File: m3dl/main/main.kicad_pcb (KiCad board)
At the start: 2 copper layers, 40 x 40 mm, 40 parts, among them IC1 STM32F405RxTx, IC2 MCP2562, J1 WEST TOP, J2 EAST TOP, J3 WEST BOT, J4 EAST BOT, J6 MICROUSB, J7 SOUTH TOP, P1 SWD_TC, U1 MICROSD, Y1 8MHz

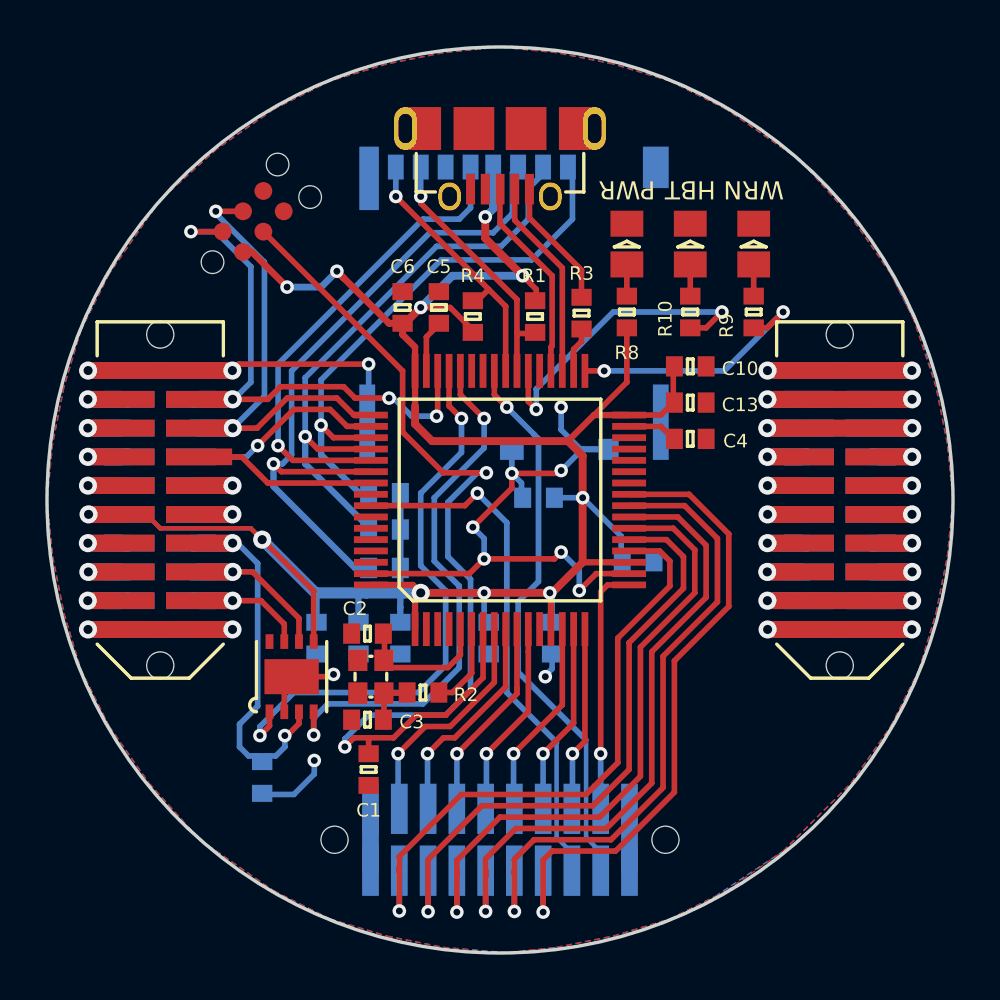
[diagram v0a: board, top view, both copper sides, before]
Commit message: Almost ready to generate gerbers
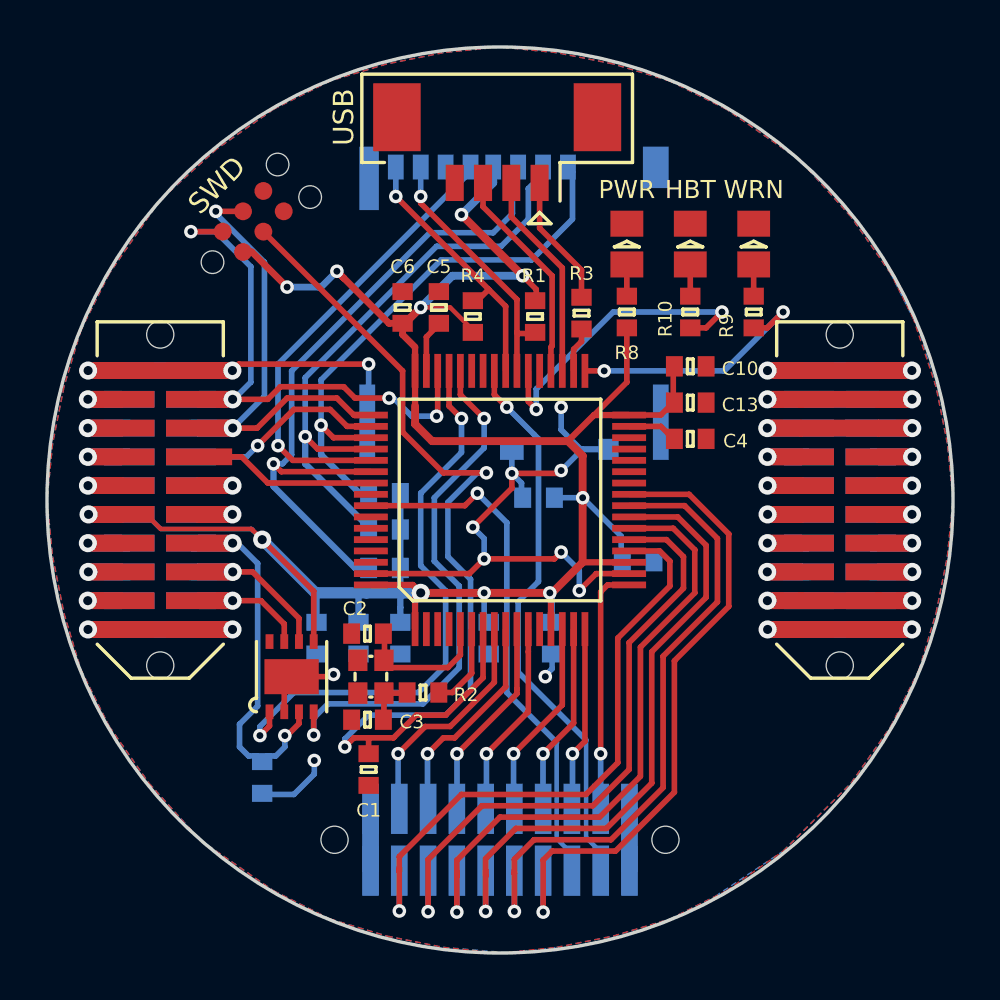
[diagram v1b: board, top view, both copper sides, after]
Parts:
- J6: value MICROUSB -> USB; footprint agg:MICROUSB_MOLEX_47589-0001 -> Connectors_Molex:Connector_Molex_PicoBlade_53261-0471
- moved J6 0.52 mm to (99.9, 83.1)
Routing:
- net 3v3: track 115.3 -> 118.4 mm
- net /SDIO_CK: track 21.3 -> 20.2 mm
- net /TEMP_INT: track 23.4 -> 24.2 mm
- net /OTG_HS_DP: track 9.00 -> 9.58 mm
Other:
- net class Default: clearance 0.1 -> 0.127; trace_width 0.25 -> 0.2
- rule pad_to_mask_clearance: 0.2 -> 0
- rule trace_clearance: 0.1 -> 0.127
- board text added: "SWD"
- board text added: "USB"
